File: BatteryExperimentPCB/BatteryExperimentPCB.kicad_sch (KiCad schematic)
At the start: 32 parts, among them J1 USB_C_Receptacle_USB2.0_14P, J2 Conn_01x12_Pin, J3 Conn_01x12_Pin, Q1 DMG1012T, SW1 SW_Push, U1 ATtiny3226-M, U2 USBLC6-2P6, U3 BQ25628RYKR

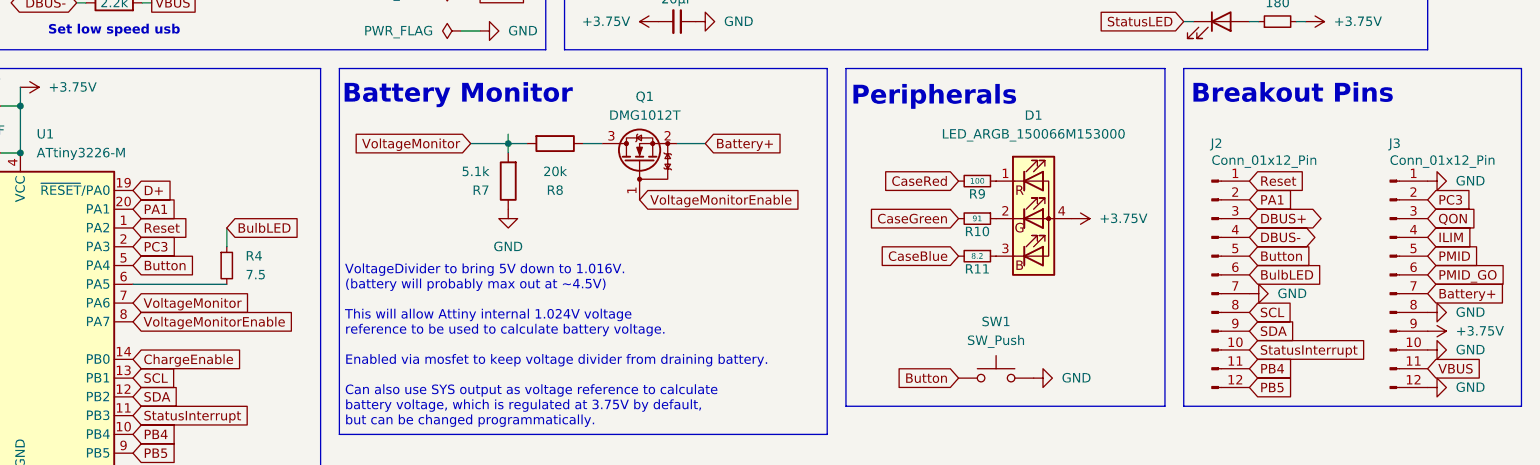
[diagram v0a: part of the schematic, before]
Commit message: more pcb work
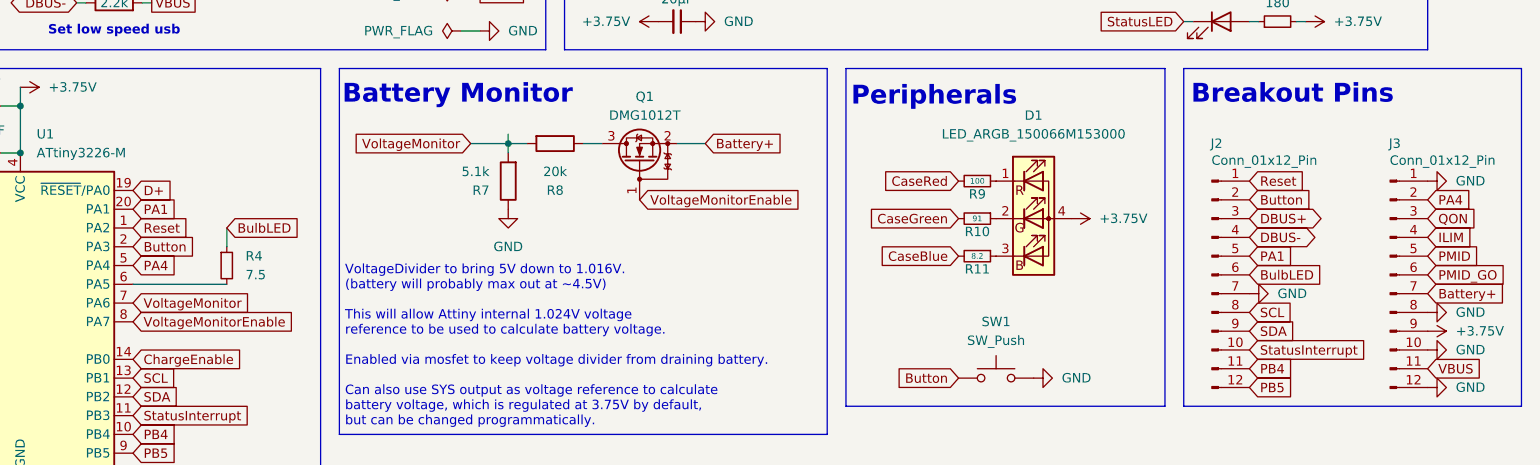
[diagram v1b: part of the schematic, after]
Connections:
- net Button: now also J2.2 (Pin_2), U1.2 (PA3); no longer J2.5 (Pin_5), U1.5 (PA4)
- net PA1: now also J2.5 (Pin_5); no longer J2.2 (Pin_2)
- net PC3 renamed PA4
- net PA4: now also U1.5 (PA4); no longer U1.2 (PA3)
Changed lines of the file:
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@@
-		)
-	)
-	(global_label "Button"
-		(shape input)
-		(at 59.69 105.41 0)
-		(fields_autoplaced yes)
-		(effects
-			(font
-				(size 1.27 1.27)
-			)
-			(justify left)
-		)
-		(property "Intersheetrefs" "${INTERSHEET_REFS}"
-			(at 68.8436 105.41 0)
-			(effects
-				(font
-					(size 1.27 1.27)
-				)
-				(justify left)
-				(hide yes)
-			)
 		)
 	)
@@
 		)
 	)
-	(global_label "PC3"
+	(global_label "PA4"
 		(shape input)
 		(at 234.95 96.52 0)
@@
 		)
 		(property "Intersheetrefs" "${INTERSHEET_REFS}"
-			(at 241.6847 96.52 0)
+			(at 241.5033 96.52 0)
 			(effects
 				(font
@@
 		)
 	)
+	(global_label "PA4"
+		(shape input)
+		(at 59.69 105.41 0)
+		(fields_autoplaced yes)
+		(effects
+			(font
+				(size 1.27 1.27)
+			)
+			(justify left)
+		)
+		(property "Intersheetrefs" "${INTERSHEET_REFS}"
+			(at 66.2433 105.41 0)
+			(effects
+				(font
+					(size 1.27 1.27)
+				)
+				(justify left)
+				(hide yes)
+			)
+		)
+	)
+	(global_label "SDA"
+		(shape input)
+		(at 210.82 31.75 180)
+		(fields_autoplaced yes)
+		(effects
+			(font
+				(size 1.27 1.27)
+			)
+			(justify right)
+		)
+		(property "Intersheetrefs" "${INTERSHEET_REFS}"
+			(at 204.2667 31.75 0)
+			(effects
+				(font
+					(size 1.27 1.27)
+				)
+				(justify right)
+				(hide yes)
+			)
+		)
+	)
 	(global_label "PA1"
 		(shape input)
-		(at 210.82 96.52 0)
-		(fields_autoplaced yes)
-		(effects
-			(font
-				(size 1.27 1.27)
-			)
-			(justify left)
-		)
-		(property "Intersheetrefs" "${INTERSHEET_REFS}"
-			(at 217.3733 96.52 0)
-			(effects
-				(font
-					(size 1.27 1.27)
-				)
-				(justify left)
-				(hide yes)
-			)
-		)
-	)
-	(global_label "SDA"
-		(shape input)
-		(at 210.82 31.75 180)
-		(fields_autoplaced yes)
-		(effects
-			(font
-				(size 1.27 1.27)
-			)
-			(justify right)
-		)
-		(property "Intersheetrefs" "${INTERSHEET_REFS}"
-			(at 204.2667 31.75 0)
-			(effects
-				(font
-					(size 1.27 1.27)
-				)
-				(justify right)
+		(at 210.82 104.14 0)
+		(fields_autoplaced yes)
+		(effects
+			(font
+				(size 1.27 1.27)
+			)
+			(justify left)
+		)
+		(property "Intersheetrefs" "${INTERSHEET_REFS}"
+			(at 217.3733 104.14 0)
+			(effects
+				(font
+					(size 1.27 1.27)
+				)
+				(justify left)
 				(hide yes)
 			)
@@
 		)
 	)
+	(global_label "Button"
+		(shape input)
+		(at 210.82 96.52 0)
+		(fields_autoplaced yes)
+		(effects
+			(font
+				(size 1.27 1.27)
+			)
+			(justify left)
+		)
+		(property "Intersheetrefs" "${INTERSHEET_REFS}"
+			(at 219.9736 96.52 0)
+			(effects
+				(font
+					(size 1.27 1.27)
+				)
+				(justify left)
+				(hide yes)
+			)
+		)
+	)
 	(global_label "CaseBlue"
 		(shape input)
@@
 		)
 	)
-	(global_label "Button"
-		(shape input)
-		(at 210.82 104.14 0)
-		(fields_autoplaced yes)
-		(effects
-			(font
-				(size 1.27 1.27)
-			)
-			(justify left)
-		)
-		(property "Intersheetrefs" "${INTERSHEET_REFS}"
-			(at 219.9736 104.14 0)
-			(effects
-				(font
-					(size 1.27 1.27)
-				)
-				(justify left)
-				(hide yes)
-			)
-		)
-	)
-	(global_label "PC3"
-		(shape input)
-		(at 59.69 102.87 0)
-		(fields_autoplaced yes)
-		(effects
-			(font
-				(size 1.27 1.27)
-			)
-			(justify left)
-		)
-		(property "Intersheetrefs" "${INTERSHEET_REFS}"
-			(at 66.4247 102.87 0)
-			(effects
-				(font
-					(size 1.27 1.27)
-				)
-				(justify left)
-				(hide yes)
-			)
-		)
-	)
 	(global_label "Battery+"
 		(shape input)
@@
 			(effects
 				(font
+					(size 1.27 1.27)
+				)
+				(justify left)
+				(hide yes)
+			)
+		)
+	)
+	(global_label "Button"
+		(shape input)
+		(at 59.69 102.87 0)
+		(fields_autoplaced yes)
+		(effects
+			(font
+				(size 1.27 1.27)
+			)
+			(justify left)
+		)
+		(property "Intersheetrefs" "${INTERSHEET_REFS}"
+			(at 68.8436 102.87 0)
+			(effects
+				(font
